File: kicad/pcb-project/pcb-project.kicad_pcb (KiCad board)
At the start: 2 copper layers, 45.7 x 35.6 mm, 13 parts, among them J1 LOGIC CONN, U1 74HC237

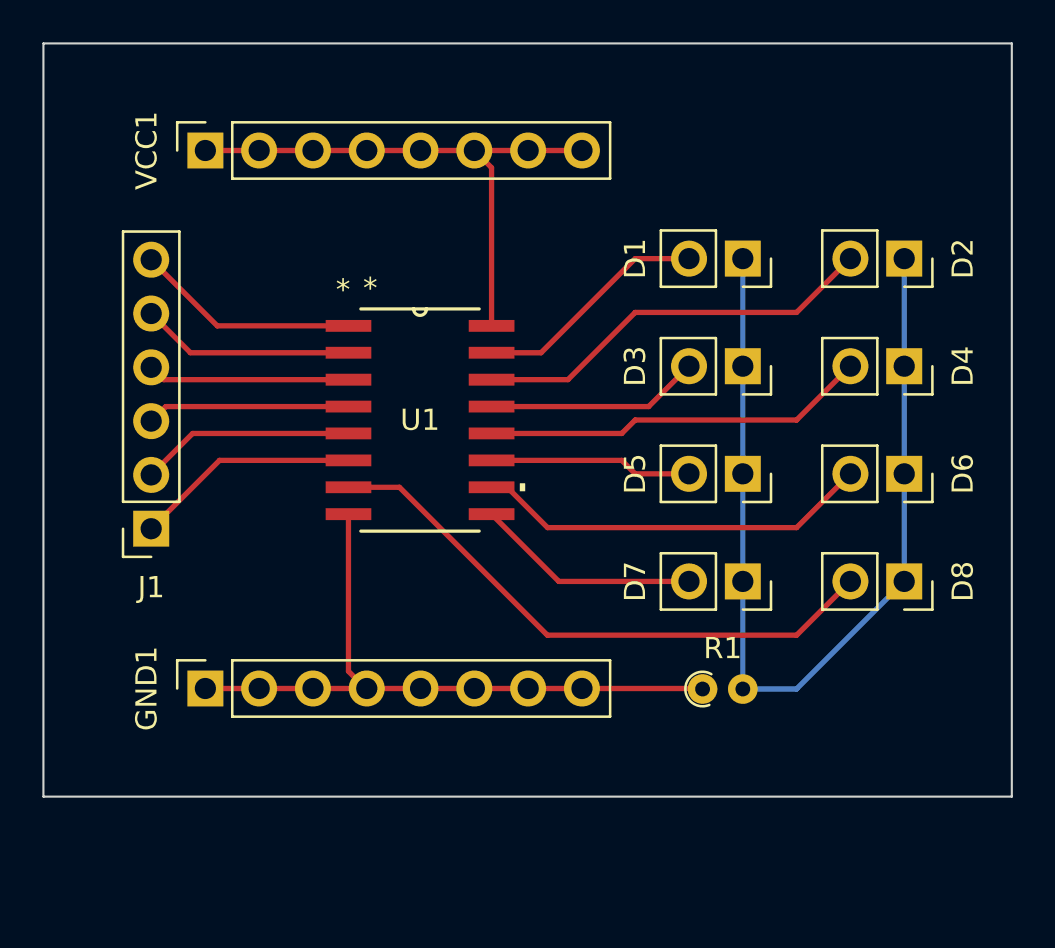
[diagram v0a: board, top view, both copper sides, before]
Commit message: finish pcb
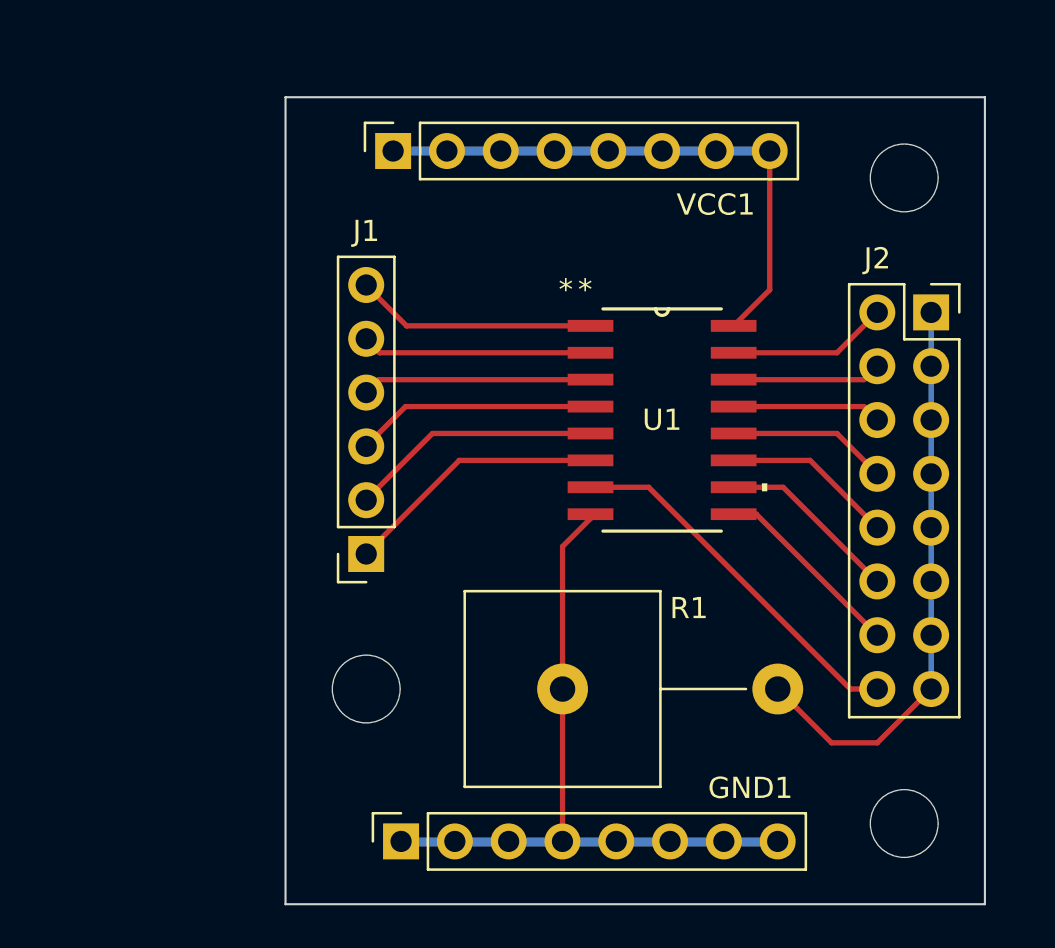
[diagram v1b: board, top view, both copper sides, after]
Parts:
- removed D1, D2, D3, D5, D6, D7: 2V, Connector_PinSocket_2.54mm:PinSocket_1x02_P2.54mm_Vertical
- removed D4, D8: 3V, Connector_PinSocket_2.54mm:PinSocket_1x02_P2.54mm_Vertical
- added H1: MountingHole, MountingHole:MountingHole_3.2mm_M3, F.Cu at (127.0, 129.5)
- added H2: MountingHole, MountingHole:MountingHole_3.2mm_M3, F.Cu at (152.4, 105.4)
- added H3: MountingHole, MountingHole:MountingHole_3.2mm_M3, F.Cu at (152.4, 135.9)
- added J2: 2-3V LEDS, Connector_PinSocket_2.54mm:PinSocket_2x08_P2.54mm_Vertical, F.Cu at (153.7, 111.8)
- R1: footprint Resistor_THT:R_Axial_DIN0204_L3.6mm_D1.6mm_P1.90mm_Vertical -> Resistor_THT:R_Axial_Power_L25.0mm_W9.0mm_P10.16mm_Vertical
- moved GND1 11.7 mm to (128.6, 136.7)
- moved U1 11.4 mm to (141.0, 116.8)
- moved J1 10.2 mm to (127.0, 123.2)
- moved VCC1 8.87 mm to (128.3, 104.1)
- moved R1 6.61 mm to (136.3, 129.5)
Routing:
- net Net-(J2-Pad1): track 45.3 -> 27.1 mm
- net Net-(J2-Pad4): track 19.3 -> 7.04 mm
- net Net-(J2-Pad8): track 18.3 -> 7.57 mm
- net Net-(J2-Pad16): track 27.6 -> 17.5 mm
- net Net-(J2-Pad12): track 18.8 -> 8.62 mm
- net Net-(J2-Pad2): track 11.2 -> 7.57 mm
- net Net-(J2-Pad6): track 10.1 -> 7.04 mm
- net Net-(J1-Pad1): track 10.7 -> 12.4 mm
- net Net-(J1-Pad3): track 9.60 -> 11.4 mm
- net Net-(J1-Pad2): track 10.1 -> 11.9 mm
- net Net-(GND1-Pad1): track 32.1 -> 33.8 mm
- net Net-(J2-Pad14): track 10.6 -> 9.15 mm
- net Net-(J2-Pad10): track 9.58 -> 8.10 mm
- net Net-(J1-Pad4): track 9.56 -> 10.9 mm
- net Net-(J1-Pad6): track 10.6 -> 11.4 mm
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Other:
- board size 45.7 x 35.6 mm -> 33 x 38.1 mm
